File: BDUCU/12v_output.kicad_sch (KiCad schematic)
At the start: 0 parts

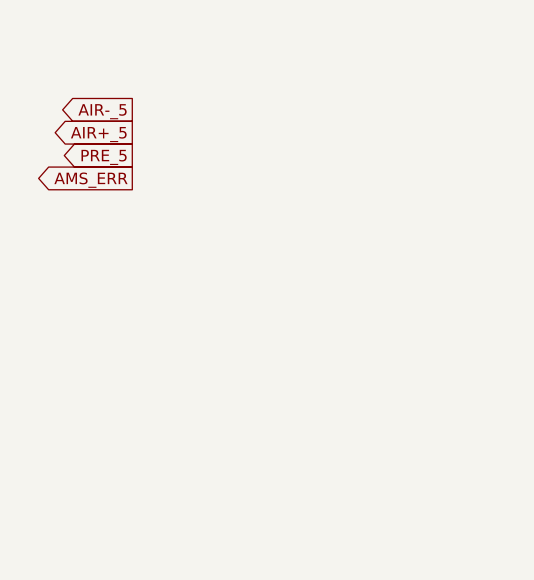
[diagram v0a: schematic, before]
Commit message: BDUCU did stuffs
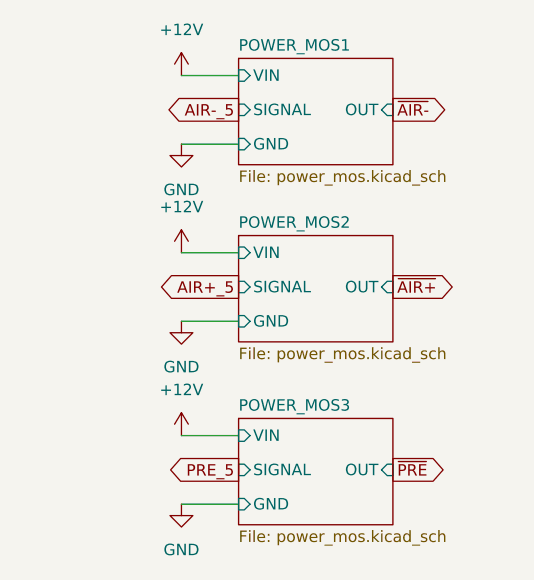
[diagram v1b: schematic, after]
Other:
- added sheet POWER_MOS1 (power_mos.kicad_sch)
- added sheet POWER_MOS2 (power_mos.kicad_sch)
- added sheet POWER_MOS3 (power_mos.kicad_sch)
